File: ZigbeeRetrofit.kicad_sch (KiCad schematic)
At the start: 23 parts, among them J1 110990030, J2 U.FL-R-SMT-1(10), J3 TC2050-IDC-NL, U1 CC2531F256RHAT, U2 SPX3819M5-L-3-3, Y1 32 Mhz, Y2 32.768 khz

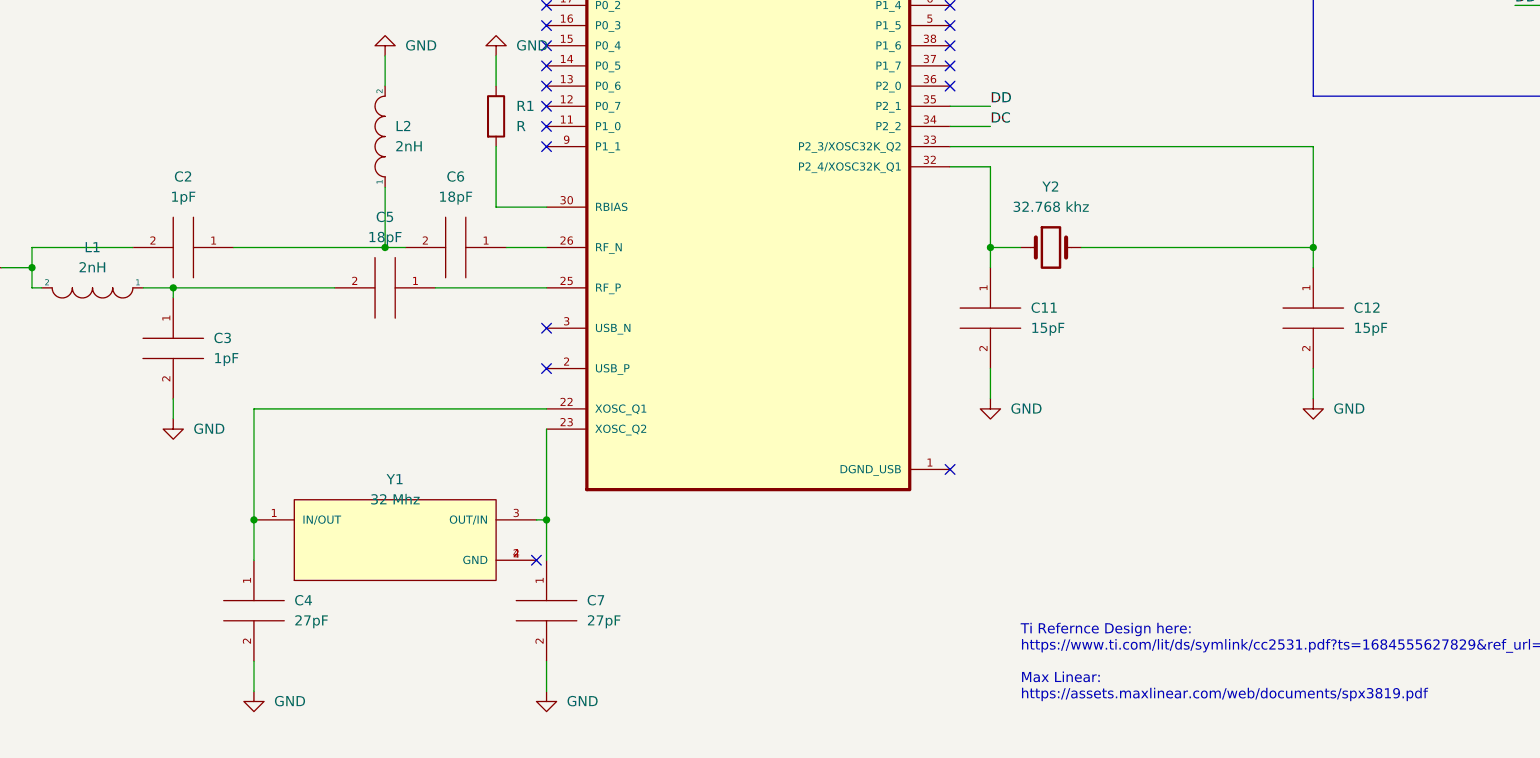
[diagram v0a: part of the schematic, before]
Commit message: Updated crystals
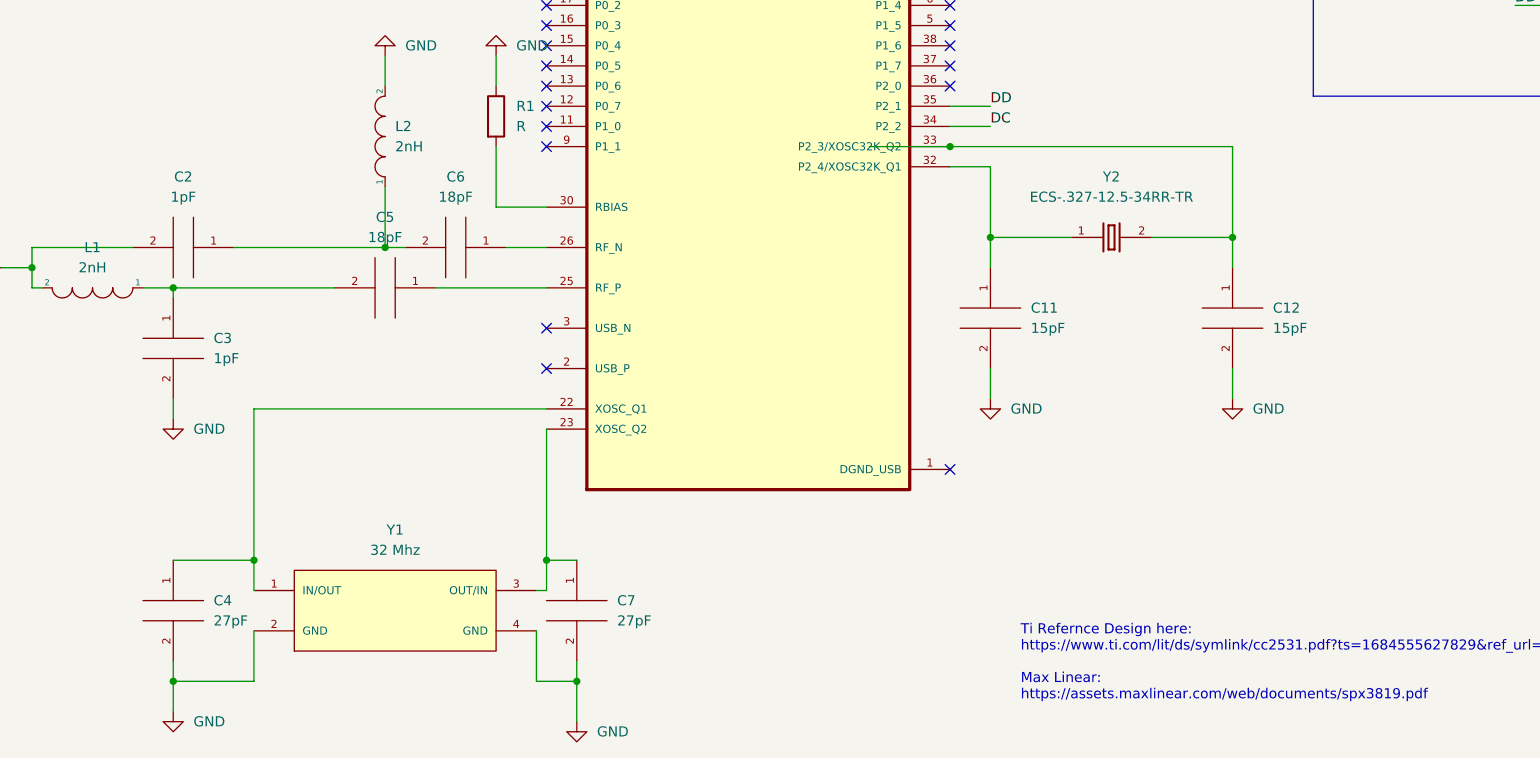
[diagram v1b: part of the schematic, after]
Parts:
- removed Y2: 32.768 khz, symbol Device:Crystal
- added Y2: ECS-.327-12.5-34RR-TR, ECS-.327-12:XTAL_ECS-.327-12.5-34RR-TR, symbol ECS-.327-12.5-34RR-TR:ECS-.327-12.5-34RR-TR
- Y1: footprint XTAL_ECS-320-13-42-CKM-TR -> ECS-320-13-42-CKM-TR:XTAL_ECS-320-13-42-CKM-TR
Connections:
- net GND: now also Y1.2 (GND), Y1.4 (GND)
- net at C11.1, U1.32 (P2_4/XOSC32K_Q1): now also Y2.1
- net at C12.1, U1.33 (P2_3/XOSC32K_Q2): now also Y2.2
- no-connect marks 28 -> 27
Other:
- moved on the sheet: C12, C4, C7
